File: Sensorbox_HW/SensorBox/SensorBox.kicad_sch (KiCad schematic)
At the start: 77 parts, among them U1 BME280, U11 PS1-O3-100, U12 DS3231M, U13 OPA197xD, U2 OPA197xD, U3 HPP845E131R5, U4 MC33063AD, U5 OPA197xD, U6 MAX31855EASA

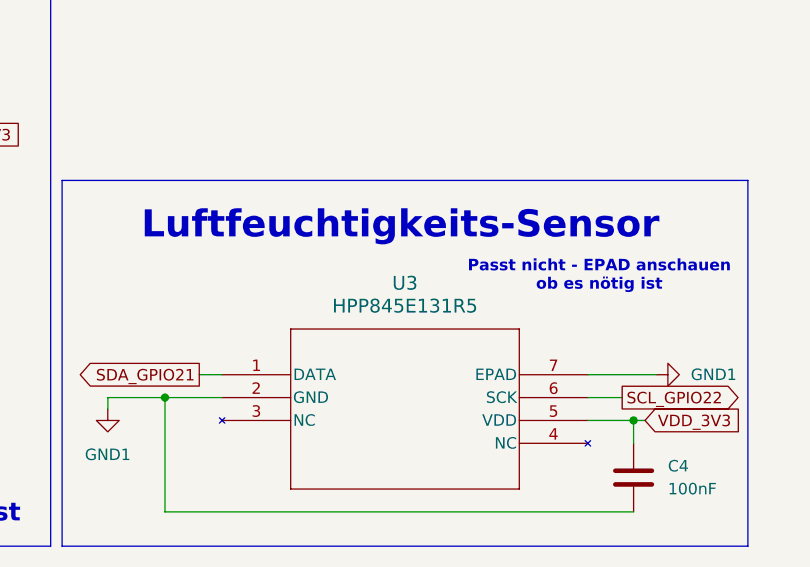
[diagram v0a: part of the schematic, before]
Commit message: PCB
Footprints zuweisen
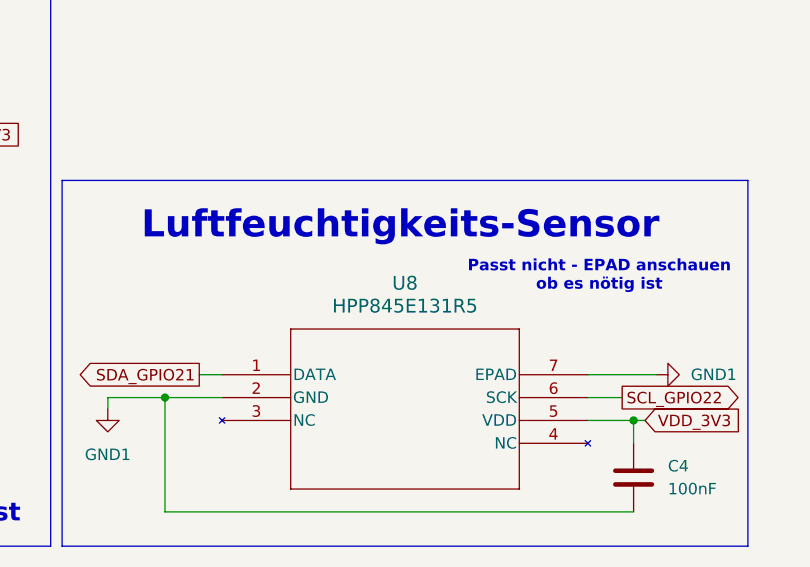
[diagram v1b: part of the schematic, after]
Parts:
- removed U3: HPP845E131R5, HPP_footprints:SON6_HPP845E131R5_TEC, symbol 2024-10-21_12-55-34:HPP845E131R5
- added U8: HPP845E131R5, HPP_footprints:SON6_HPP845E131R5_TEC, symbol 2024-10-21_12-55-34:HPP845E131R5
- BT1: footprint Battery:BatteryHolder_Keystone_2479_3xAAA -> Battery_Basket:BatteryHolder_Keystone_2479_3xAAA
- F1: footprint (none) -> Fuse:Fuse_Littelfuse_372_D8.50mm
- JP1: footprint (none) -> Connector_PinHeader_2.54mm:PinHeader_1x02_P2.54mm_Vertical
- R1_2: footprint Resistor_SMD:R_0402_1005Metric -> Resistor_THT:R_Axial_DIN0204_L3.6mm_D1.6mm_P7.62mm_Horizontal
- U1: footprint Package_LGA:Bosch_LGA-8_2.5x2.5mm_P0.65mm_ClockwisePinNumbering -> BME280 (2):BME280
- U11: footprint PS1O3100 -> Ozonsensor:PS1O3100
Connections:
- net GND1: now also U8.2 (GND), U8.7 (EPAD)
- net SCL_GPIO22: now also U8.6 (SCK)
- net SDA_GPIO21: now also U8.1 (DATA)
- net VDD_3V3: now also U8.5 (VDD)
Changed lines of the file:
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@@
 			)
 		)
-		(property "Footprint" "Battery:BatteryHolder_Keystone_2479_3xAAA"
+		(property "Footprint" "Battery_Basket:BatteryHolder_Keystone_2479_3xAAA"
 			(at 128.27 54.61 0)
 			(effects
@@
 			)
 		)
-		(property "Footprint" "Resistor_SMD:R_0402_1005Metric"
+		(property "Footprint" "Resistor_THT:R_Axial_DIN0204_L3.6mm_D1.6mm_P7.62mm_Horizontal"
 			(at 177.8 235.712 90)
 			(effects
@@
 			)
 		)
-		(property "Footprint" ""
+		(property "Footprint" "Fuse:Fuse_Littelfuse_372_D8.50mm"
 			(at 147.32 43.18 0)
 			(effects
@@
 	)
 	(symbol
-		(lib_id "2024-10-21_12-55-34:HPP845E131R5")
-		(at 95.25 170.18 0)
-		(unit 1)
-		(exclude_from_sim no)
-		(in_bom yes)
-		(on_board yes)
-		(dnp no)
-		(fields_autoplaced yes)
-		(property "Reference" "U3"
-			(at 115.57 160.02 0)
-			(effects
-				(font
-					(size 1.524 1.524)
-				)
-			)
-		)
-		(property "Value" "HPP845E131R5"
-			(at 115.57 162.56 0)
-			(effects
-				(font
-					(size 1.524 1.524)
-				)
-			)
-		)
-		(property "Footprint" "HPP_footprints:SON6_HPP845E131R5_TEC"
-			(at 95.25 170.18 0)
-			(effects
-				(font
-					(size 1.27 1.27)
-					(italic yes)
-				)
-				(hide yes)
-			)
-		)
-		(property "Datasheet" "HPP845E131R5"
-			(at 95.25 170.18 0)
-			(effects
-				(font
-					(size 1.27 1.27)
-					(italic yes)
-				)
-				(hide yes)
-			)
-		)
-		(property "Description" ""
-			(at 95.25 170.18 0)
-			(effects
-				(font
-					(size 1.27 1.27)
-				)
-				(hide yes)
-			)
-		)
-		(pin "2"
-		)
-		(pin "1"
-		)
-		(pin "7"
-		)
-		(pin "5"
-		)
-		(pin "3"
-		)
-		(pin "4"
-		)
-		(pin "6"
-		)
-		(instances
-			(project "SensorBox"
-				(path "/7cbe8151-7294-42e6-9c4e-6ec8952d674f"
-					(reference "U3")
-					(unit 1)
-				)
-			)
-		)
-	)
-	(symbol
 		(lib_id "Device:R")
 		(at 36.83 34.29 0)
@@
 			)
 		)
-		(property "Footprint" "PS1O3100"
+		(property "Footprint" "Ozonsensor:PS1O3100"
 			(at 115.57 146.38 0)
 			(effects
@@
 			)
 		)
-		(property "Footprint" ""
+		(property "Footprint" "Connector_PinHeader_2.54mm:PinHeader_1x02_P2.54mm_Vertical"
 			(at 294.64 214.63 0)
 			(effects
@@
 	)
 	(symbol
+		(lib_id "2024-10-21_12-55-34:HPP845E131R5")
+		(at 95.25 170.18 0)
+		(unit 1)
+		(exclude_from_sim no)
+		(in_bom yes)
+		(on_board yes)
+		(dnp no)
+		(fields_autoplaced yes)
+		(property "Reference" "U8"
+			(at 115.57 160.02 0)
+			(effects
+				(font
+					(size 1.524 1.524)
+				)
+			)
+		)
+		(property "Value" "HPP845E131R5"
+			(at 115.57 162.56 0)
+			(effects
+				(font
+					(size 1.524 1.524)
+				)
+			)
+		)
+		(property "Footprint" "HPP_footprints:SON6_HPP845E131R5_TEC"
+			(at 95.25 170.18 0)
+			(effects
+				(font
+					(size 1.27 1.27)
+					(italic yes)
+				)
+				(hide yes)
+			)
+		)
+		(property "Datasheet" "HPP845E131R5"
+			(at 95.25 170.18 0)
+			(effects
+				(font
+					(size 1.27 1.27)
+					(italic yes)
+				)
+				(hide yes)
+			)
+		)
+		(property "Description" ""
+			(at 95.25 170.18 0)
+			(effects
+				(font
+					(size 1.27 1.27)
+				)
+				(hide yes)
+			)
+		)
+		(pin "6"
+		)
+		(pin "2"
+		)
+		(pin "7"
+		)
+		(pin "4"
+		)
+		(pin "3"
+		)
+		(pin "1"
+		)
+		(pin "5"
+		)
+		(instances
+			(project ""
+				(path "/7cbe8151-7294-42e6-9c4e-6ec8952d674f"
+					(reference "U8")
+					(unit 1)
+				)
+			)
+		)
+	)
+	(symbol
 		(lib_id "Sensor_Temperature:MAX31855EASA")
 		(at 289.56 190.5 90)
@@
 			)
 		)
-		(property "Footprint" "Package_LGA:Bosch_LGA-8_2.5x2.5mm_P0.65mm_ClockwisePinNumbering"
+		(property "Footprint" "BME280 (2):BME280"
 			(at 22.86 179.07 0)
 			(effects
